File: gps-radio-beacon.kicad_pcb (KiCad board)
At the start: 2 copper layers, 106.4 x 69.7 mm, 40 parts, among them J1 Conn_01x16, J2 Conn_01x16, J3 Conn_Coaxial, J4 Conn_Coaxial, J5 Screw_Terminal_01x04, P1 USB_C_Plug_USB2.0, Q1 Q_PMOS_DGS, U1 PGA2040, U2 RFM95W-915S2, U3 MAX-M10S, U4 NCP1117-3.3_SOT223

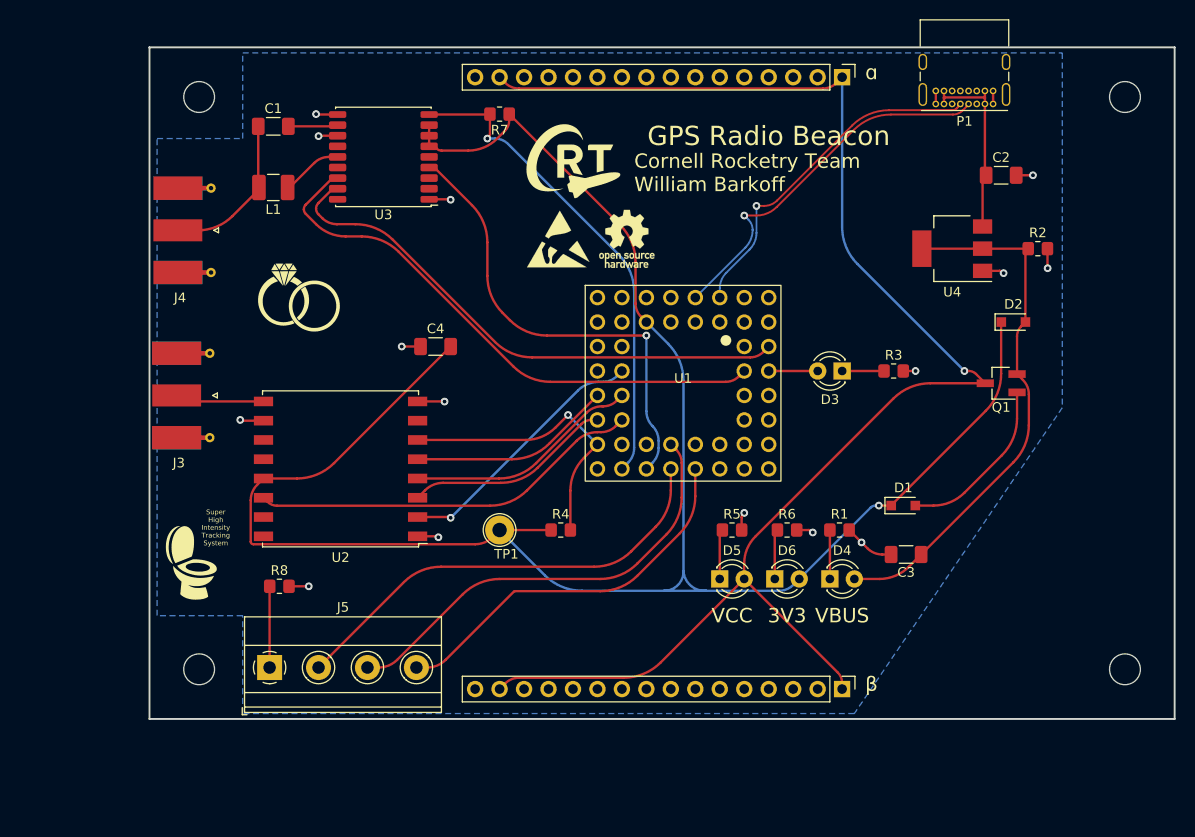
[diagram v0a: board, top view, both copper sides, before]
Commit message: Revert "update silkscreen"
This reverts commit 1eaeaa331c0a90a38e124b6b08bc37b13ba27824.
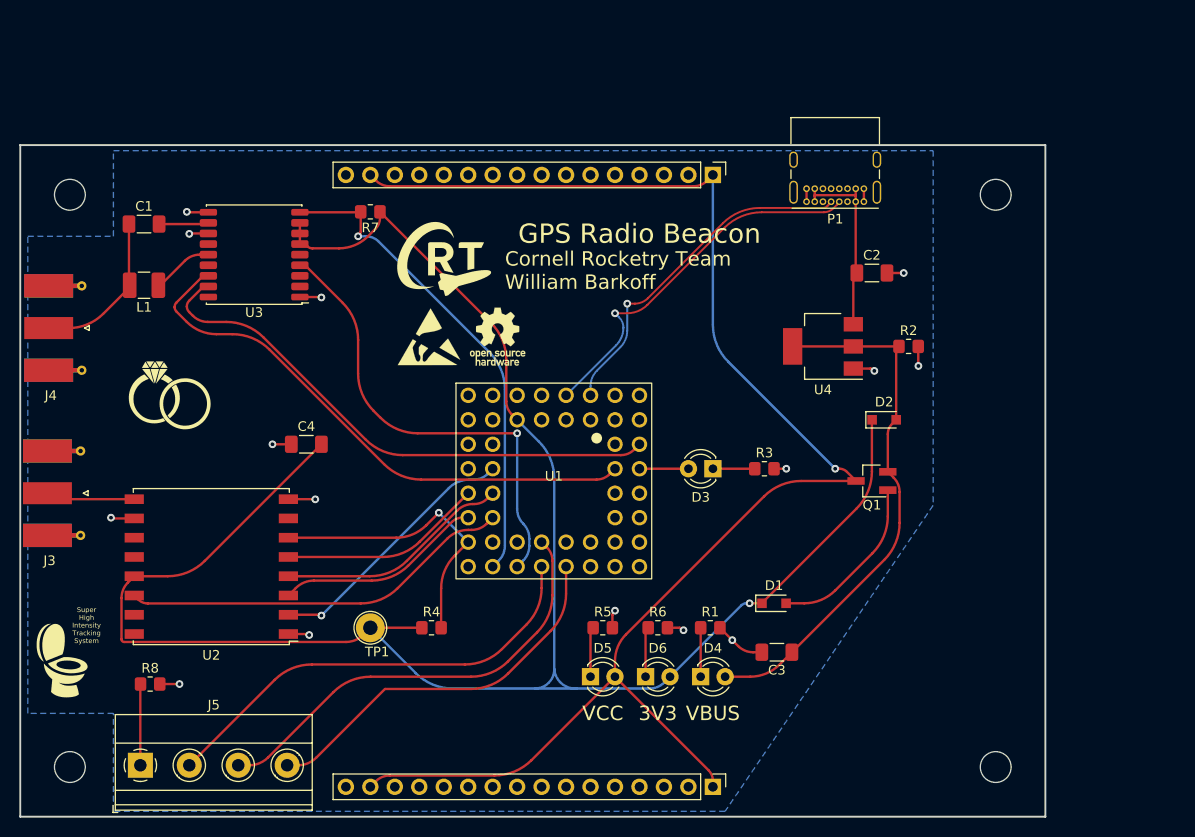
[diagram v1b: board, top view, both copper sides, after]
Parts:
- moved C3 16.8 mm to (161.6, 128.3)
- moved J2 16.8 mm to (154.9, 142.2)
- moved C2 16.8 mm to (171.4, 88.9)
- moved C4 16.8 mm to (112.7, 106.7)
- moved D1 16.8 mm to (161.3, 123.2)
- moved D2 16.8 mm to (172.7, 104.1)
- moved D3 16.8 mm to (154.9, 109.2)
- moved D4 16.8 mm to (153.7, 130.8)
- moved D6 16.8 mm to (147.9, 130.8)
- moved G*** 16.8 mm to (127.0, 87.4)
- moved G*** 16.8 mm to (87.4, 129.3)
- moved H1 16.8 mm to (88.2, 80.8)
- moved H2 16.8 mm to (184.3, 80.8)
- moved J1 16.8 mm to (154.9, 78.7)
- moved J3 16.8 mm to (87.6, 111.8)
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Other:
- board text added: "REV YYYY-MM-DD"
- board text removed: "REV 0.2.0"
- board text removed: "ɑ"
- board text removed: "β"

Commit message: update silkscreen
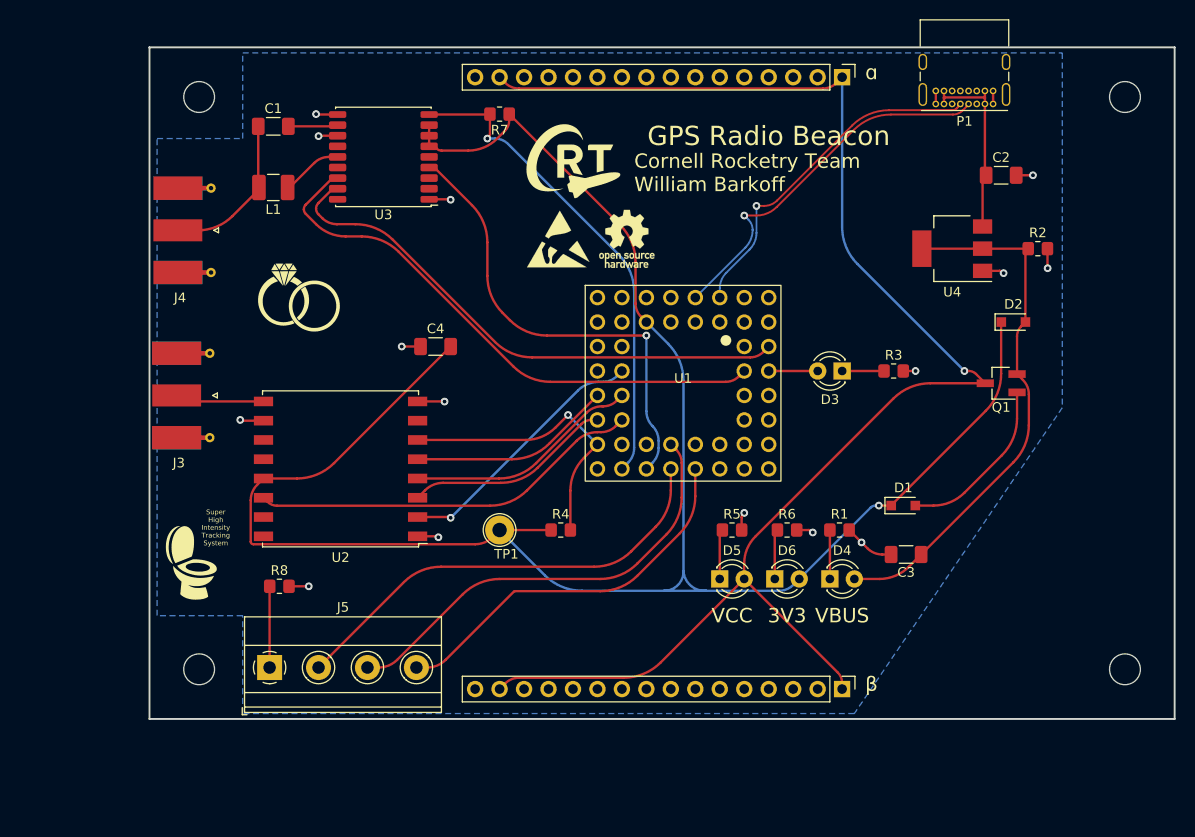
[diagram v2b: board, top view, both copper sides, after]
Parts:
- moved C3 16.8 mm to (175.0, 118.1)
- moved J2 16.8 mm to (168.4, 132.1)
- moved C2 16.8 mm to (184.9, 78.8)
- moved C4 16.8 mm to (126.2, 96.5)
- moved D1 16.8 mm to (174.7, 113.0)
- moved D2 16.8 mm to (186.1, 94.0)
- moved D3 16.8 mm to (168.4, 99.1)
- moved D4 16.8 mm to (167.1, 120.7)
- moved D6 16.8 mm to (161.4, 120.7)
- moved G*** 16.8 mm to (140.4, 77.2)
- moved G*** 16.8 mm to (100.8, 119.1)
- moved H1 16.8 mm to (101.6, 70.6)
- moved H2 16.8 mm to (197.7, 70.6)
- moved J1 16.8 mm to (168.4, 68.6)
- moved J3 16.8 mm to (101.0, 101.6)
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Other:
- board text added: "REV 0.2.0"
- board text added: "ɑ"
- board text added: "β"
- board text removed: "REV YYYY-MM-DD"
